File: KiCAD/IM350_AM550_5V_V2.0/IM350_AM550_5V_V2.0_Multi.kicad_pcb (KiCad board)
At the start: 2 copper layers, 100 x 99 mm, 130 parts, among them J5 USB_B_Micro_Power, J7 RJ12, P3 0R, P4 0R, SW1 Pairing, U1 MCP1700-3302E_SOT23, U2 ESP-12F

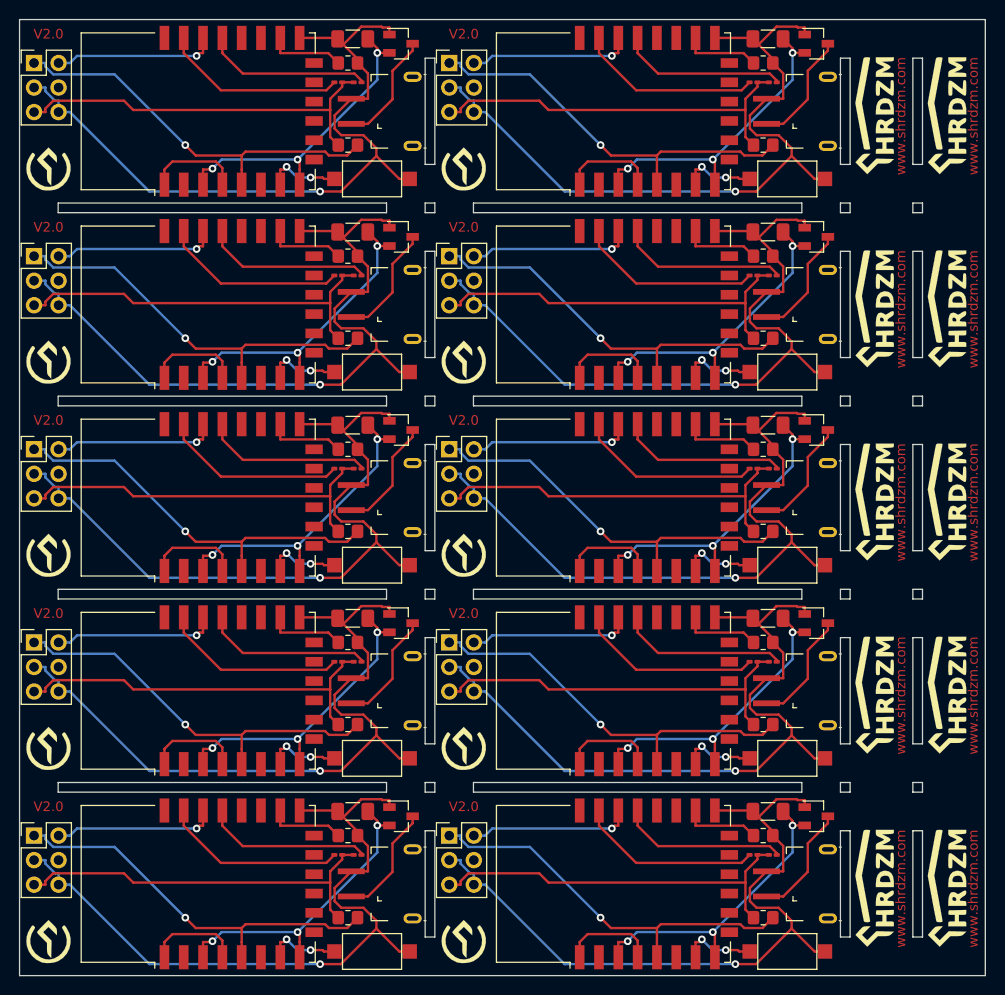
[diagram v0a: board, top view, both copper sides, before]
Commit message: Update
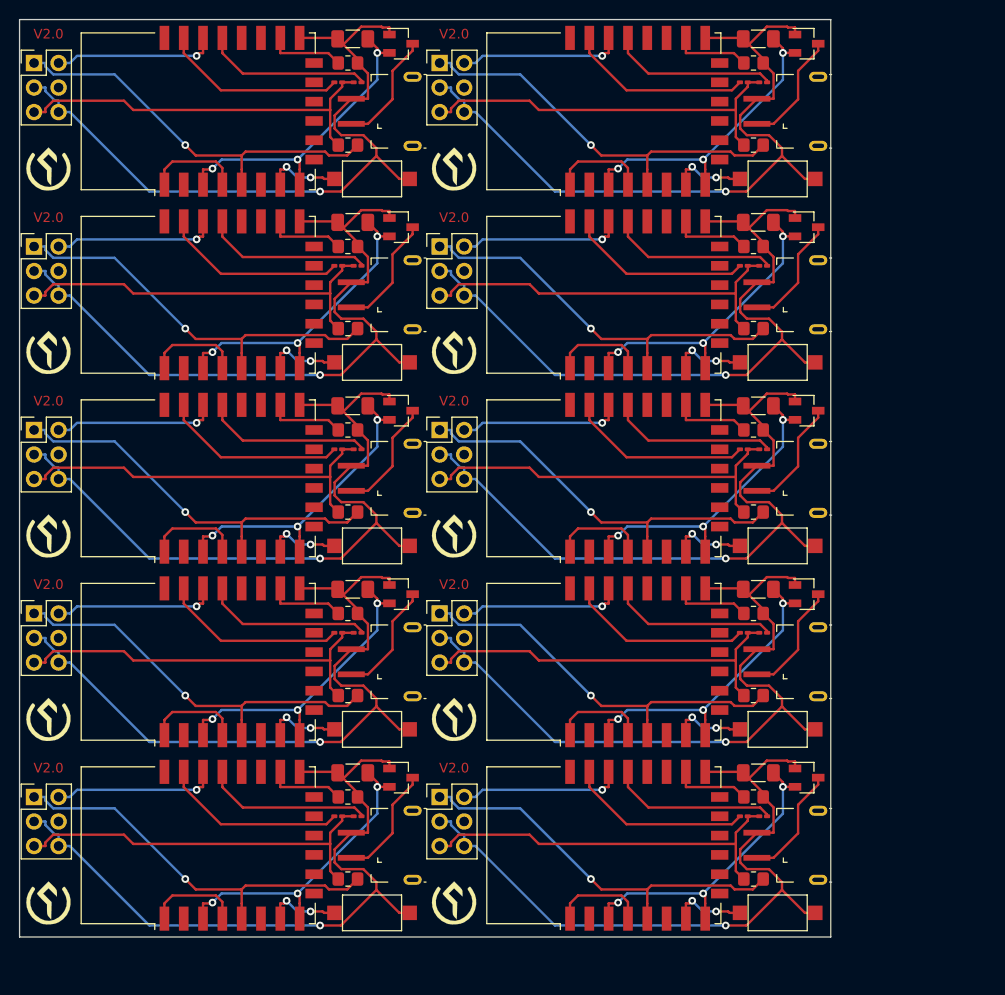
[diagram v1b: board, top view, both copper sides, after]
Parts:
- removed the C2 at (63.0, 106.5)
- removed the C2 at (106.0, 106.5)
- removed the C2 at (63.0, 86.5)
- removed the C2 at (106.0, 86.5)
- removed the C2 at (63.0, 66.5)
- removed the C2 at (106.0, 66.5)
- removed the C2 at (63.0, 46.5)
- removed the C2 at (106.0, 46.5)
- removed the C2 at (106.0, 26.5)
- removed G*** (x10): LOGO, SHRDZM:SHRDZM 12x4
- removed the G1 at (74.5, 120.0)
- removed the G1 at (31.5, 120.0)
- removed the G1 at (31.5, 100.0)
- removed the G1 at (74.5, 100.0)
- removed the G1 at (31.5, 80.0)
- removed the G1 at (74.5, 80.0)
- removed the G1 at (31.5, 60.0)
- removed the G1 at (74.5, 60.0)
- removed the G1 at (74.5, 40.0)
- removed the G2 at (51.0, 111.5)
- removed the G2 at (94.0, 111.5)
- removed the G2 at (51.0, 91.5)
- removed the G2 at (94.0, 91.5)
- removed the G2 at (51.0, 71.5)
- removed the G2 at (94.0, 71.5)
- removed the G2 at (51.0, 51.5)
- removed the G2 at (94.0, 51.5)
- removed the G2 at (94.0, 31.5)
- removed the J5 at (111.0, 114.0)
- removed the J5 at (68.0, 114.0)
- removed the J5 at (68.0, 94.0)
- removed the J5 at (111.0, 94.0)
- removed the J5 at (68.0, 74.0)
- removed the J5 at (111.0, 74.0)
- removed the J5 at (68.0, 54.0)
- removed the J5 at (111.0, 54.0)
- removed the J5 at (111.0, 34.0)
- removed the J7 at (73.0, 109.0)
- removed the J7 at (30.0, 109.0)
- removed the J7 at (73.0, 89.0)
- removed the J7 at (30.0, 89.0)
- removed the J7 at (30.0, 69.0)
- removed the J7 at (73.0, 69.0)
- removed the J7 at (30.0, 49.0)
- removed the J7 at (73.0, 49.0)
- removed the J7 at (73.0, 29.0)
- removed the P3 at (104.5, 111.0)
- removed the P3 at (61.5, 111.0)
- removed the P3 at (104.5, 91.0)
- removed the P3 at (61.5, 91.0)
- removed the P3 at (61.5, 71.0)
- removed the P3 at (104.5, 71.0)
- removed the P3 at (61.5, 51.0)
- removed the P3 at (104.5, 51.0)
- removed the P3 at (104.5, 31.0)
- removed the P4 at (106.5, 111.0)
- removed the P4 at (63.5, 111.0)
- removed the P4 at (106.5, 91.0)
- removed the P4 at (63.5, 91.0)
- removed the P4 at (106.5, 71.0)
- removed the P4 at (63.5, 71.0)
- removed the P4 at (63.5, 51.0)
- removed the P4 at (106.5, 51.0)
- removed the P4 at (106.5, 31.0)
- removed the R1 at (62.5, 109.0)
- removed the R1 at (105.5, 109.0)
- removed the R1 at (62.5, 89.0)
- removed the R1 at (105.5, 89.0)
- removed the R1 at (62.5, 69.0)
- removed the R1 at (105.5, 69.0)
- removed the R1 at (62.5, 49.0)
- removed the R1 at (105.5, 49.0)
- removed the R1 at (105.5, 29.0)
- removed the R5 at (105.5, 117.5)
- removed the R5 at (62.5, 117.5)
- removed the R5 at (105.5, 97.5)
- removed the R5 at (62.5, 97.5)
- removed the R5 at (62.5, 77.5)
- removed the R5 at (105.5, 77.5)
- removed the R5 at (62.5, 57.5)
- removed the R5 at (105.5, 57.5)
- removed the R5 at (105.5, 37.5)
- removed the SW1 at (65.0, 121.0)
- removed the SW1 at (108.0, 121.0)
- removed the SW1 at (108.0, 101.0)
- removed the SW1 at (65.0, 101.0)
- removed the SW1 at (65.0, 81.0)
- removed the SW1 at (108.0, 81.0)
- removed the SW1 at (65.0, 61.0)
- removed the SW1 at (108.0, 61.0)
- removed the SW1 at (108.0, 41.0)
- removed the U1 at (68.0, 107.0)
- removed the U1 at (111.0, 107.0)
- removed the U1 at (68.0, 87.0)
- removed the U1 at (111.0, 87.0)
- removed the U1 at (68.0, 67.0)
- removed the U1 at (111.0, 67.0)
- removed the U1 at (68.0, 47.0)
- removed the U1 at (111.0, 47.0)
- removed the U1 at (111.0, 27.0)
- removed the U2 at (90.0, 114.0)
- removed the U2 at (47.0, 114.0)
- removed the U2 at (47.0, 94.0)
- removed the U2 at (90.0, 94.0)
- removed the U2 at (47.0, 74.0)
- removed the U2 at (90.0, 74.0)
- removed the U2 at (47.0, 54.0)
- removed the U2 at (90.0, 54.0)
- removed the U2 at (90.0, 34.0)
- added C2: 100nF, Capacitor_SMD:C_1206_3216Metric_Pad1.33x1.80mm_HandSolder, F.Cu at (63.0, 102.5)
- added C2: 100nF, Capacitor_SMD:C_1206_3216Metric_Pad1.33x1.80mm_HandSolder, F.Cu at (105.0, 102.5)
- added C2: 100nF, Capacitor_SMD:C_1206_3216Metric_Pad1.33x1.80mm_HandSolder, F.Cu at (105.0, 83.5)
- added C2: 100nF, Capacitor_SMD:C_1206_3216Metric_Pad1.33x1.80mm_HandSolder, F.Cu at (63.0, 83.5)
- added C2: 100nF, Capacitor_SMD:C_1206_3216Metric_Pad1.33x1.80mm_HandSolder, F.Cu at (63.0, 64.5)
- added C2: 100nF, Capacitor_SMD:C_1206_3216Metric_Pad1.33x1.80mm_HandSolder, F.Cu at (105.0, 64.5)
- added C2: 100nF, Capacitor_SMD:C_1206_3216Metric_Pad1.33x1.80mm_HandSolder, F.Cu at (105.0, 45.5)
- added C2: 100nF, Capacitor_SMD:C_1206_3216Metric_Pad1.33x1.80mm_HandSolder, F.Cu at (63.0, 45.5)
- added C2: 100nF, Capacitor_SMD:C_1206_3216Metric_Pad1.33x1.80mm_HandSolder, F.Cu at (105.0, 26.5)
- added G1: LOGO, SHRDZM:SHRDZM Symbol 5x5, F.Cu at (73.5, 116.0)
- added G1: LOGO, SHRDZM:SHRDZM Symbol 5x5, F.Cu at (31.5, 116.0)
- added G1: LOGO, SHRDZM:SHRDZM Symbol 5x5, F.Cu at (73.5, 97.0)
- added G1: LOGO, SHRDZM:SHRDZM Symbol 5x5, F.Cu at (31.5, 97.0)
- added G1: LOGO, SHRDZM:SHRDZM Symbol 5x5, F.Cu at (31.5, 78.0)
- added G1: LOGO, SHRDZM:SHRDZM Symbol 5x5, F.Cu at (73.5, 78.0)
- added G1: LOGO, SHRDZM:SHRDZM Symbol 5x5, F.Cu at (73.5, 59.0)
- added G1: LOGO, SHRDZM:SHRDZM Symbol 5x5, F.Cu at (31.5, 59.0)
- added G1: LOGO, SHRDZM:SHRDZM Symbol 5x5, F.Cu at (73.5, 40.0)
- added G2: LOGO, SHRDZM:SHRDZM 33x11, B.Cu at (93.0, 107.5)
- added G2: LOGO, SHRDZM:SHRDZM 33x11, B.Cu at (51.0, 107.5)
- added G2: LOGO, SHRDZM:SHRDZM 33x11, B.Cu at (93.0, 88.5)
- added G2: LOGO, SHRDZM:SHRDZM 33x11, B.Cu at (51.0, 88.5)
- added G2: LOGO, SHRDZM:SHRDZM 33x11, B.Cu at (51.0, 69.5)
- added G2: LOGO, SHRDZM:SHRDZM 33x11, B.Cu at (93.0, 69.5)
- added G2: LOGO, SHRDZM:SHRDZM 33x11, B.Cu at (93.0, 50.5)
- added G2: LOGO, SHRDZM:SHRDZM 33x11, B.Cu at (51.0, 50.5)
- added G2: LOGO, SHRDZM:SHRDZM 33x11, B.Cu at (93.0, 31.5)
- added J5: USB_B_Micro_Power, SHRDZM:USB_Micro-B_Power, F.Cu at (68.0, 110.0)
- added J5: USB_B_Micro_Power, SHRDZM:USB_Micro-B_Power, F.Cu at (110.0, 110.0)
- added J5: USB_B_Micro_Power, SHRDZM:USB_Micro-B_Power, F.Cu at (110.0, 91.0)
- added J5: USB_B_Micro_Power, SHRDZM:USB_Micro-B_Power, F.Cu at (68.0, 91.0)
- added J5: USB_B_Micro_Power, SHRDZM:USB_Micro-B_Power, F.Cu at (68.0, 72.0)
- added J5: USB_B_Micro_Power, SHRDZM:USB_Micro-B_Power, F.Cu at (110.0, 72.0)
- added J5: USB_B_Micro_Power, SHRDZM:USB_Micro-B_Power, F.Cu at (110.0, 53.0)
- added J5: USB_B_Micro_Power, SHRDZM:USB_Micro-B_Power, F.Cu at (68.0, 53.0)
- added J5: USB_B_Micro_Power, SHRDZM:USB_Micro-B_Power, F.Cu at (110.0, 34.0)
- added J7: RJ12, Connector_PinHeader_2.54mm:PinHeader_2x03_P2.54mm_Vertical, F.Cu at (30.0, 105.0)
- added J7: RJ12, Connector_PinHeader_2.54mm:PinHeader_2x03_P2.54mm_Vertical, F.Cu at (72.0, 105.0)
- added J7: RJ12, Connector_PinHeader_2.54mm:PinHeader_2x03_P2.54mm_Vertical, F.Cu at (72.0, 86.0)
- added J7: RJ12, Connector_PinHeader_2.54mm:PinHeader_2x03_P2.54mm_Vertical, F.Cu at (30.0, 86.0)
- added J7: RJ12, Connector_PinHeader_2.54mm:PinHeader_2x03_P2.54mm_Vertical, F.Cu at (30.0, 67.0)
- added J7: RJ12, Connector_PinHeader_2.54mm:PinHeader_2x03_P2.54mm_Vertical, F.Cu at (72.0, 67.0)
- added J7: RJ12, Connector_PinHeader_2.54mm:PinHeader_2x03_P2.54mm_Vertical, F.Cu at (72.0, 48.0)
- added J7: RJ12, Connector_PinHeader_2.54mm:PinHeader_2x03_P2.54mm_Vertical, F.Cu at (30.0, 48.0)
- added J7: RJ12, Connector_PinHeader_2.54mm:PinHeader_2x03_P2.54mm_Vertical, F.Cu at (72.0, 29.0)
- added P3: 0R, Resistor_SMD:R_0201_0603Metric_Pad0.64x0.40mm_HandSolder, F.Cu at (103.5, 107.0)
- added P3: 0R, Resistor_SMD:R_0201_0603Metric_Pad0.64x0.40mm_HandSolder, F.Cu at (61.5, 107.0)
- added P3: 0R, Resistor_SMD:R_0201_0603Metric_Pad0.64x0.40mm_HandSolder, F.Cu at (103.5, 88.0)
- added P3: 0R, Resistor_SMD:R_0201_0603Metric_Pad0.64x0.40mm_HandSolder, F.Cu at (61.5, 88.0)
- added P3: 0R, Resistor_SMD:R_0201_0603Metric_Pad0.64x0.40mm_HandSolder, F.Cu at (61.5, 69.0)
- added P3: 0R, Resistor_SMD:R_0201_0603Metric_Pad0.64x0.40mm_HandSolder, F.Cu at (103.5, 69.0)
- added P3: 0R, Resistor_SMD:R_0201_0603Metric_Pad0.64x0.40mm_HandSolder, F.Cu at (103.5, 50.0)
- added P3: 0R, Resistor_SMD:R_0201_0603Metric_Pad0.64x0.40mm_HandSolder, F.Cu at (61.5, 50.0)
- added P3: 0R, Resistor_SMD:R_0201_0603Metric_Pad0.64x0.40mm_HandSolder, F.Cu at (103.5, 31.0)
- added P4: 0R, Resistor_SMD:R_0201_0603Metric_Pad0.64x0.40mm_HandSolder, F.Cu at (63.5, 107.0)
- added P4: 0R, Resistor_SMD:R_0201_0603Metric_Pad0.64x0.40mm_HandSolder, F.Cu at (105.5, 107.0)
- added P4: 0R, Resistor_SMD:R_0201_0603Metric_Pad0.64x0.40mm_HandSolder, F.Cu at (105.5, 88.0)
- added P4: 0R, Resistor_SMD:R_0201_0603Metric_Pad0.64x0.40mm_HandSolder, F.Cu at (63.5, 88.0)
- added P4: 0R, Resistor_SMD:R_0201_0603Metric_Pad0.64x0.40mm_HandSolder, F.Cu at (63.5, 69.0)
- added P4: 0R, Resistor_SMD:R_0201_0603Metric_Pad0.64x0.40mm_HandSolder, F.Cu at (105.5, 69.0)
- added P4: 0R, Resistor_SMD:R_0201_0603Metric_Pad0.64x0.40mm_HandSolder, F.Cu at (105.5, 50.0)
- added P4: 0R, Resistor_SMD:R_0201_0603Metric_Pad0.64x0.40mm_HandSolder, F.Cu at (63.5, 50.0)
- added P4: 0R, Resistor_SMD:R_0201_0603Metric_Pad0.64x0.40mm_HandSolder, F.Cu at (105.5, 31.0)
- added R1: 10k, Resistor_SMD:R_0805_2012Metric_Pad1.20x1.40mm_HandSolder, F.Cu at (62.5, 105.0)
- added R1: 10k, Resistor_SMD:R_0805_2012Metric_Pad1.20x1.40mm_HandSolder, F.Cu at (104.5, 105.0)
- added R1: 10k, Resistor_SMD:R_0805_2012Metric_Pad1.20x1.40mm_HandSolder, F.Cu at (104.5, 86.0)
- added R1: 10k, Resistor_SMD:R_0805_2012Metric_Pad1.20x1.40mm_HandSolder, F.Cu at (62.5, 86.0)
- added R1: 10k, Resistor_SMD:R_0805_2012Metric_Pad1.20x1.40mm_HandSolder, F.Cu at (62.5, 67.0)
- added R1: 10k, Resistor_SMD:R_0805_2012Metric_Pad1.20x1.40mm_HandSolder, F.Cu at (104.5, 67.0)
- added R1: 10k, Resistor_SMD:R_0805_2012Metric_Pad1.20x1.40mm_HandSolder, F.Cu at (104.5, 48.0)
- added R1: 10k, Resistor_SMD:R_0805_2012Metric_Pad1.20x1.40mm_HandSolder, F.Cu at (62.5, 48.0)
- added R1: 10k, Resistor_SMD:R_0805_2012Metric_Pad1.20x1.40mm_HandSolder, F.Cu at (104.5, 29.0)
- added R5: 10k, Resistor_SMD:R_0805_2012Metric_Pad1.20x1.40mm_HandSolder, F.Cu at (62.5, 113.5)
- added R5: 10k, Resistor_SMD:R_0805_2012Metric_Pad1.20x1.40mm_HandSolder, F.Cu at (104.5, 113.5)
- added R5: 10k, Resistor_SMD:R_0805_2012Metric_Pad1.20x1.40mm_HandSolder, F.Cu at (104.5, 94.5)
- added R5: 10k, Resistor_SMD:R_0805_2012Metric_Pad1.20x1.40mm_HandSolder, F.Cu at (62.5, 94.5)
- added R5: 10k, Resistor_SMD:R_0805_2012Metric_Pad1.20x1.40mm_HandSolder, F.Cu at (62.5, 75.5)
- added R5: 10k, Resistor_SMD:R_0805_2012Metric_Pad1.20x1.40mm_HandSolder, F.Cu at (104.5, 75.5)
- added R5: 10k, Resistor_SMD:R_0805_2012Metric_Pad1.20x1.40mm_HandSolder, F.Cu at (104.5, 56.5)
- added R5: 10k, Resistor_SMD:R_0805_2012Metric_Pad1.20x1.40mm_HandSolder, F.Cu at (62.5, 56.5)
- added R5: 10k, Resistor_SMD:R_0805_2012Metric_Pad1.20x1.40mm_HandSolder, F.Cu at (104.5, 37.5)
- added SW1: Pairing, Button_Switch_SMD:SW_SPST_CK_RS282G05A3, F.Cu at (107.0, 117.0)
- added SW1: Pairing, Button_Switch_SMD:SW_SPST_CK_RS282G05A3, F.Cu at (65.0, 117.0)
- added SW1: Pairing, Button_Switch_SMD:SW_SPST_CK_RS282G05A3, F.Cu at (107.0, 98.0)
- added SW1: Pairing, Button_Switch_SMD:SW_SPST_CK_RS282G05A3, F.Cu at (65.0, 98.0)
- added SW1: Pairing, Button_Switch_SMD:SW_SPST_CK_RS282G05A3, F.Cu at (65.0, 79.0)
- added SW1: Pairing, Button_Switch_SMD:SW_SPST_CK_RS282G05A3, F.Cu at (107.0, 79.0)
- added SW1: Pairing, Button_Switch_SMD:SW_SPST_CK_RS282G05A3, F.Cu at (107.0, 60.0)
- added SW1: Pairing, Button_Switch_SMD:SW_SPST_CK_RS282G05A3, F.Cu at (65.0, 60.0)
- added SW1: Pairing, Button_Switch_SMD:SW_SPST_CK_RS282G05A3, F.Cu at (107.0, 41.0)
- added U1: MCP1700-3302E_SOT23, ErichCollection:SOT-23_Handsoldering, F.Cu at (68.0, 103.0)
- added U1: MCP1700-3302E_SOT23, ErichCollection:SOT-23_Handsoldering, F.Cu at (110.0, 103.0)
- added U1: MCP1700-3302E_SOT23, ErichCollection:SOT-23_Handsoldering, F.Cu at (110.0, 84.0)
- added U1: MCP1700-3302E_SOT23, ErichCollection:SOT-23_Handsoldering, F.Cu at (68.0, 84.0)
- added U1: MCP1700-3302E_SOT23, ErichCollection:SOT-23_Handsoldering, F.Cu at (68.0, 65.0)
- added U1: MCP1700-3302E_SOT23, ErichCollection:SOT-23_Handsoldering, F.Cu at (110.0, 65.0)
- added U1: MCP1700-3302E_SOT23, ErichCollection:SOT-23_Handsoldering, F.Cu at (110.0, 46.0)
- added U1: MCP1700-3302E_SOT23, ErichCollection:SOT-23_Handsoldering, F.Cu at (68.0, 46.0)
- added U1: MCP1700-3302E_SOT23, ErichCollection:SOT-23_Handsoldering, F.Cu at (110.0, 27.0)
- added U2: ESP-12F, RF_Module:ESP-12E, F.Cu at (47.0, 110.0)
- added U2: ESP-12F, RF_Module:ESP-12E, F.Cu at (89.0, 110.0)
- added U2: ESP-12F, RF_Module:ESP-12E, F.Cu at (89.0, 91.0)
- added U2: ESP-12F, RF_Module:ESP-12E, F.Cu at (47.0, 91.0)
- added U2: ESP-12F, RF_Module:ESP-12E, F.Cu at (89.0, 72.0)
- added U2: ESP-12F, RF_Module:ESP-12E, F.Cu at (47.0, 72.0)
- added U2: ESP-12F, RF_Module:ESP-12E, F.Cu at (89.0, 53.0)
- added U2: ESP-12F, RF_Module:ESP-12E, F.Cu at (47.0, 53.0)
- added U2: ESP-12F, RF_Module:ESP-12E, F.Cu at (89.0, 34.0)
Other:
- board size 100 x 99 mm -> 84 x 95 mm
